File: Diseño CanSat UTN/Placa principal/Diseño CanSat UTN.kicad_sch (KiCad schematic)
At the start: 0 parts

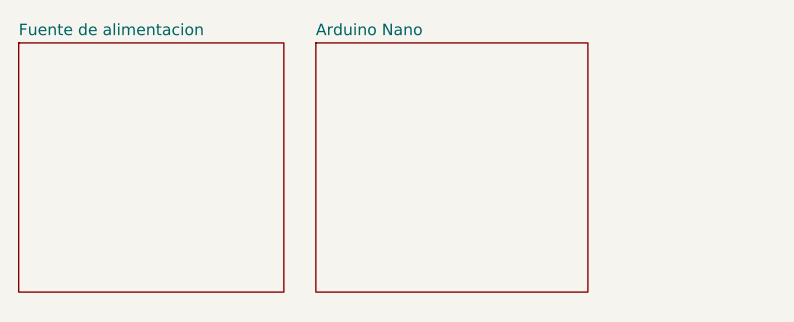
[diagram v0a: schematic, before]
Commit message: Eliminando Backups
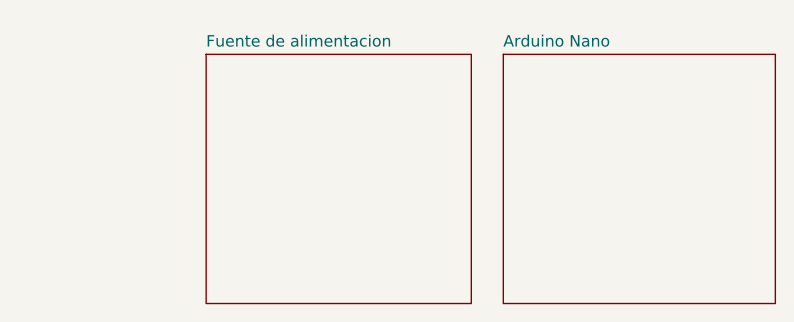
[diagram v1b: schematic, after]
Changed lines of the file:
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@@
 (kicad_sch (version 20230121) (generator eeschema)
   (paper "A5")
-  (sheet (at 48.514 50.546) (size 29.464 27.686) (fields_autoplaced)
+  (sheet (at 69.342 51.816) (size 29.464 27.686) (fields_autoplaced)
     (stroke (width 0.1524) (type solid))
     (fill (color 0 0 0 0.0000))
-    (property "Sheetname" "Fuente de alimentacion" (at 48.514 49.8344 0)
+    (property "Sheetname" "Fuente de alimentacion" (at 69.342 51.1044 0)
       (effects (font (size 1.27 1.27)) (justify left bottom))
     )
-    (property "Sheetfile" "Fuente de alimentacion.kicad_sch" (at 48.514 78.8166 0)
+    (property "Sheetfile" "Fuente de alimentacion.kicad_sch" (at 69.342 80.0866 0)
       (effects (font (size 1.27 1.27)) (justify left top) hide)
     )
@@
     )
   )
-  (sheet (at 81.534 50.546) (size 30.226 27.686) (fields_autoplaced)
+  (sheet (at 102.362 51.816) (size 30.226 27.686) (fields_autoplaced)
     (stroke (width 0.1524) (type solid))
     (fill (color 0 0 0 0.0000))
-    (property "Sheetname" "Arduino Nano" (at 81.534 49.8344 0)
+    (property "Sheetname" "Arduino Nano" (at 102.362 51.1044 0)
       (effects (font (size 1.27 1.27)) (justify left bottom))
     )
-    (property "Sheetfile" "Arduino Nano.kicad_sch" (at 81.534 78.8166 0)
+    (property "Sheetfile" "Arduino Nano.kicad_sch" (at 102.362 80.0866 0)
       (effects (font (size 1.27 1.27)) (justify left top) hide)
     )
